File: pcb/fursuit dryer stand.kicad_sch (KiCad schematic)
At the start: 3 parts, among them J1 OLED, U1 ESP32-C3, U2 BME280

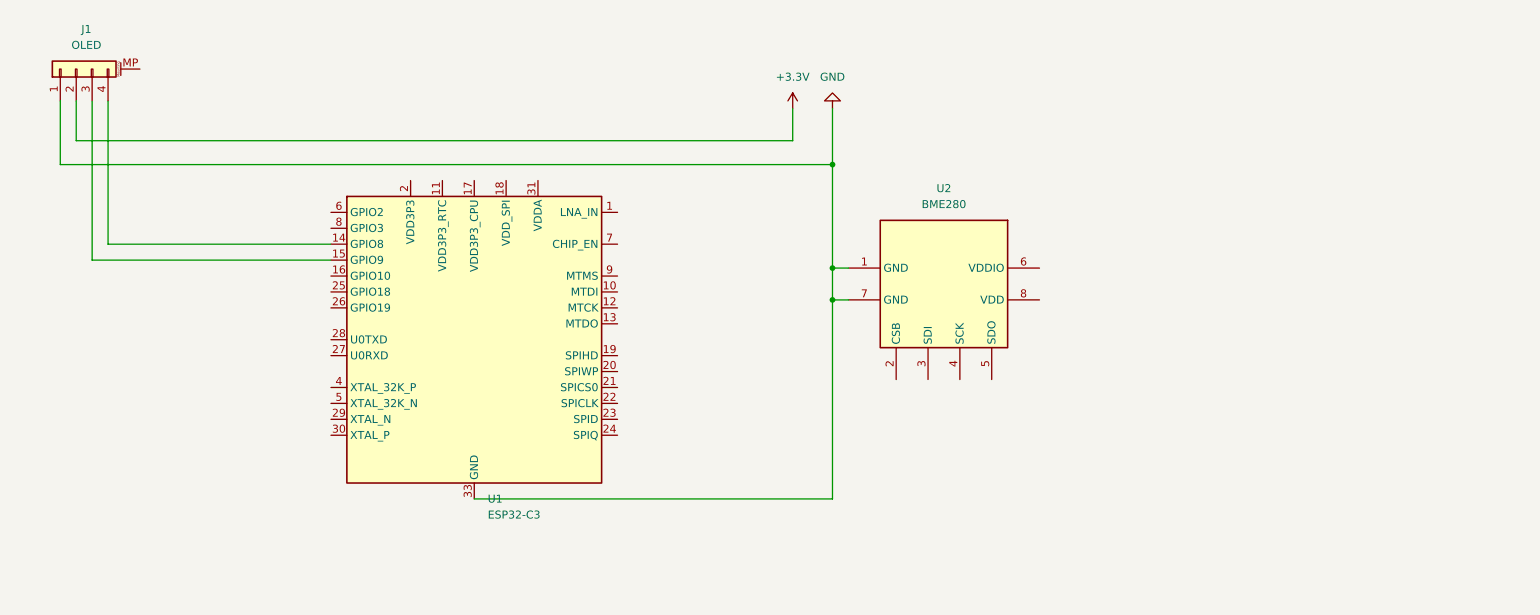
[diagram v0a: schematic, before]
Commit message: Add files via upload
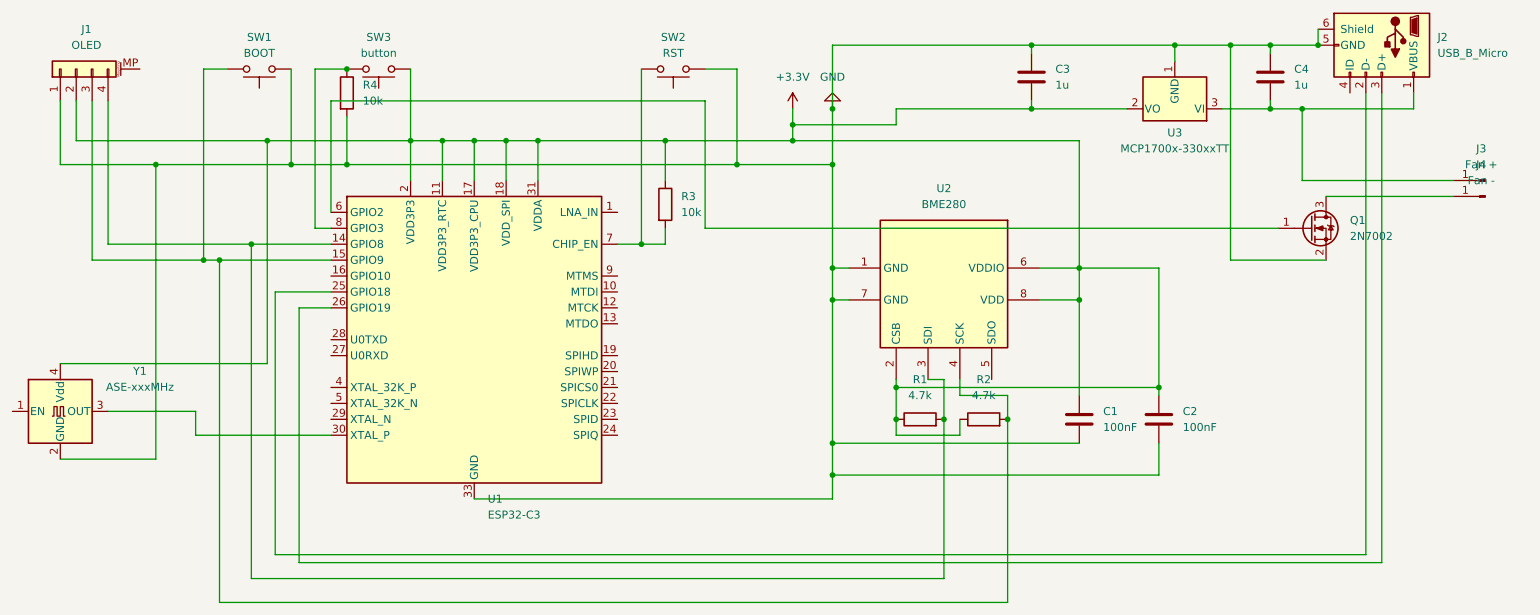
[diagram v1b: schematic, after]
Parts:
- added C1, C2: 100nF, Capacitor_SMD:C_0805_2012Metric_Pad1.18x1.45mm_HandSolder, symbol Device:C
- added C3, C4: 1u, Capacitor_SMD:C_0805_2012Metric_Pad1.18x1.45mm_HandSolder, symbol Device:C
- added J2: USB_B_Micro, Connector_USB:USB_Micro-AB_Molex_47590-0001, symbol Connector:USB_B_Micro
- added J3: Fan +, Connector_Wire:SolderWirePad_1x01_SMD_1x2mm, symbol Connector:Conn_01x01_Pin
- added J4: Fan -, Connector_Wire:SolderWirePad_1x01_SMD_1x2mm, symbol Connector:Conn_01x01_Pin
- added Q1: 2N7002, Package_TO_SOT_SMD:SOT-23, symbol Transistor_FET:2N7002
- added R1, R2: 4.7k, Resistor_SMD:R_0805_2012Metric_Pad1.20x1.40mm_HandSolder, symbol Device:R
- added R3, R4: 10k, Resistor_SMD:R_0805_2012Metric_Pad1.20x1.40mm_HandSolder, symbol Device:R
- added SW1: BOOT, Button_Switch_SMD:SW_SPST_CK_RS282G05A3, symbol Switch:SW_Push
- added SW2: RST, Button_Switch_SMD:SW_SPST_CK_RS282G05A3, symbol Switch:SW_Push
- added SW3: button, Button_Switch_SMD:SW_SPST_CK_RS282G05A3, symbol Switch:SW_Push
- added U3: MCP1700x-330xxTT, Package_TO_SOT_SMD:SOT-23, symbol Regulator_Linear:MCP1700x-330xxTT
- added Y1: ASE-xxxMHz, Crystal:Crystal_SMD_TXC_AX_8045-2Pin_8.0x4.5mm, symbol Oscillator:ASE-xxxMHz
- J1: footprint (none) -> Connector_PinSocket_2.54mm:PinSocket_1x04_P2.54mm_Vertical_SMD_Pin1Left
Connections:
- net +3.3V: now also U1.11 (VDD3P3_RTC), U1.17 (VDD3P3_CPU), U1.18 (VDD_SPI), U1.2 (VDD3P3), U1.3 (VDD3P3), U1.31 (VDDA), U1.32 (VDDA), U2.2 (CSB), U2.6 (VDDIO), U2.8 (VDD), C1.1, C2.1, C3.2, R1.1, R2.1, R3.1, SW3.1, U3.2 (VO), Y1.4 (Vdd)
- net GND: now also C1.2, C2.2, C3.1, C4.1, J2.5 (GND), J2.6 (Shield), Q1.2 (S), R4.2, SW1.1, SW2.1, U3.1 (GND), Y1.2 (GND)
- net at J1.3 (Pin_3), U1.15 (GPIO9): now also U2.4 (SCK), R2.2, SW1.2
- net at J1.4 (Pin_4), U1.14 (GPIO8): now also U2.3 (SDI), R1.2
- net at U1.25 (GPIO18): now also J2.2 (D-)
- net at U1.26 (GPIO19): now also J2.3 (D+)
- net at U1.30 (XTAL_P): now also Y1.3 (OUT)
- net at U1.6 (GPIO2): now also Q1.1 (G)
- net at U1.7 (CHIP_EN): now also R3.2, SW2.2
- net at U1.8 (GPIO3): now also R4.1, SW3.2
- new net: C4.2, J2.1 (VBUS), J3.1 (Pin_1), U3.3 (VI)
- new net: J4.1 (Pin_1), Q1.3 (D)
